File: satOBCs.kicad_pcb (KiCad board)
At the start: 2 copper layers, 55.2 x 94.2 mm, 11 parts, among them J1 Battery power, J2 Conn_01x10_Pin, J3 Conn_01x10_Pin, SW1 SW_Push, U2 mpu-9250, U3 AZ1117-3.3, U6 DHT11

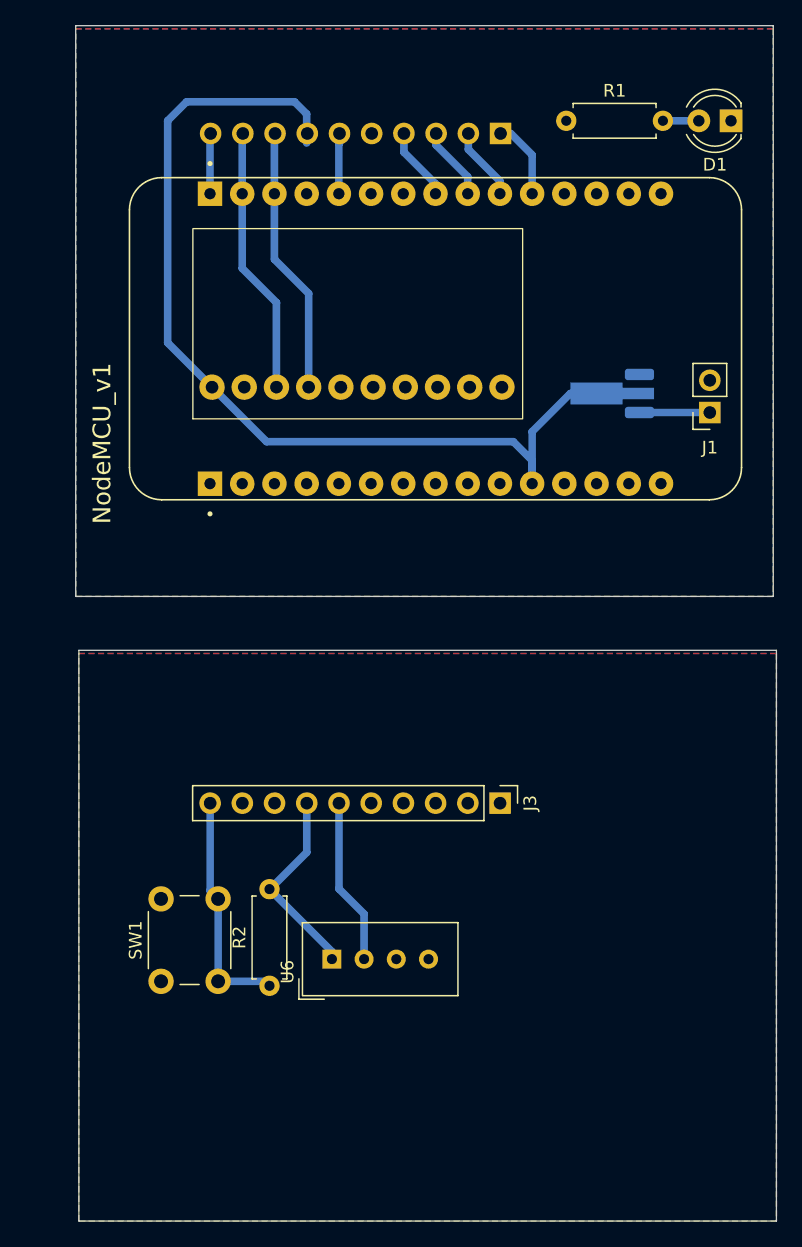
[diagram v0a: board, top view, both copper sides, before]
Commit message: 4th edited
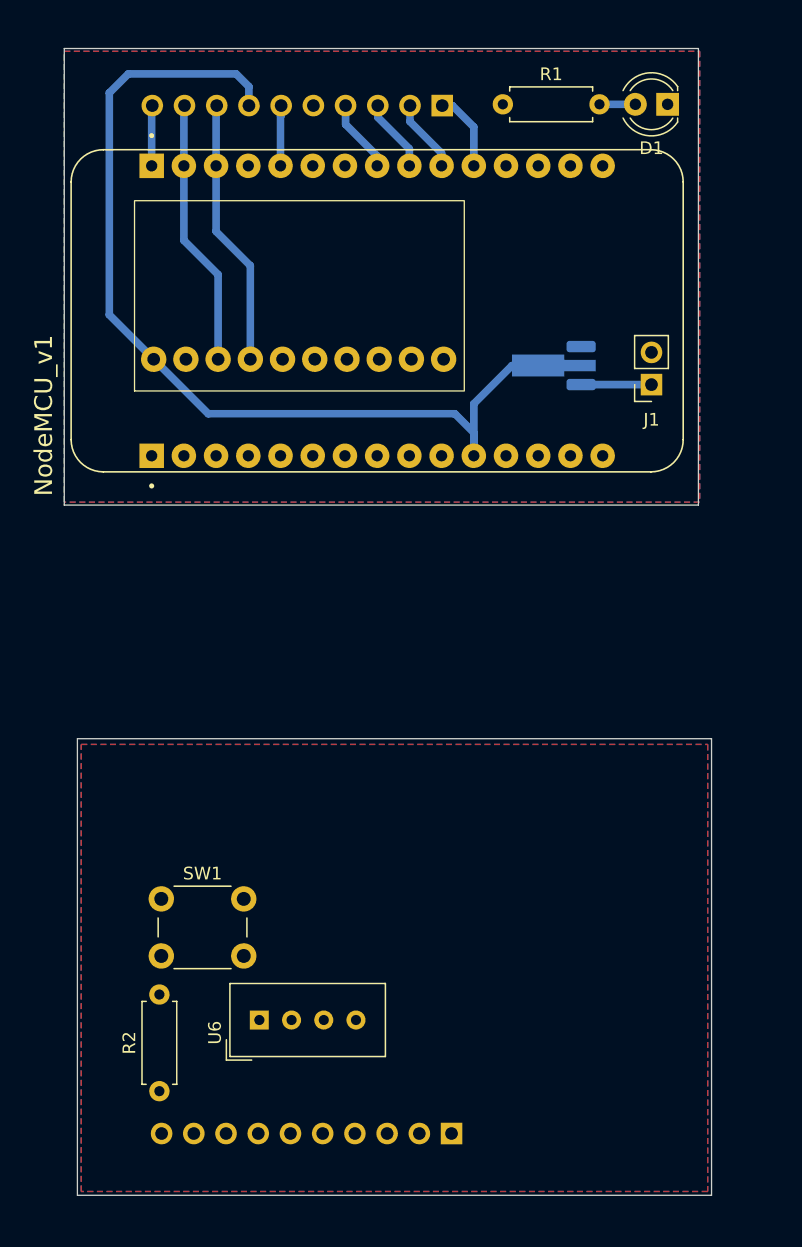
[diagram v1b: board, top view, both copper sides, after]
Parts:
- J3: moved to B.Cu
- moved J3 26.3 mm to (136.6, 133.8), turned to 90 degrees
- moved R2 12.0 mm to (113.6, 130.5)
- moved U6 7.47 mm to (121.5, 124.9)
- moved SW1 6.50 mm to (113.8, 115.3), turned to 0 degrees
- moved D1 5.17 mm to (153.7, 52.7)
- moved R1 5.17 mm to (140.7, 52.7)
- moved U2 5.10 mm to (126.1, 67.8)
- moved J1 5.10 mm to (152.4, 74.8)
- moved J2 5.10 mm to (135.9, 52.8)
- moved NodeMCU_v1 5.10 mm to (130.8, 69.0)
- moved U3 5.10 mm to (144.4, 73.3)
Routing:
- net /RST: track 22.5 -> 4.00 mm
- net +3V3: track 95.5 -> 79.2 mm
- net /DHT_data: track 17.9 -> 4.77 mm
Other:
- board size 55.2 x 94.2 mm -> 51 x 90.4 mm

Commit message: added last
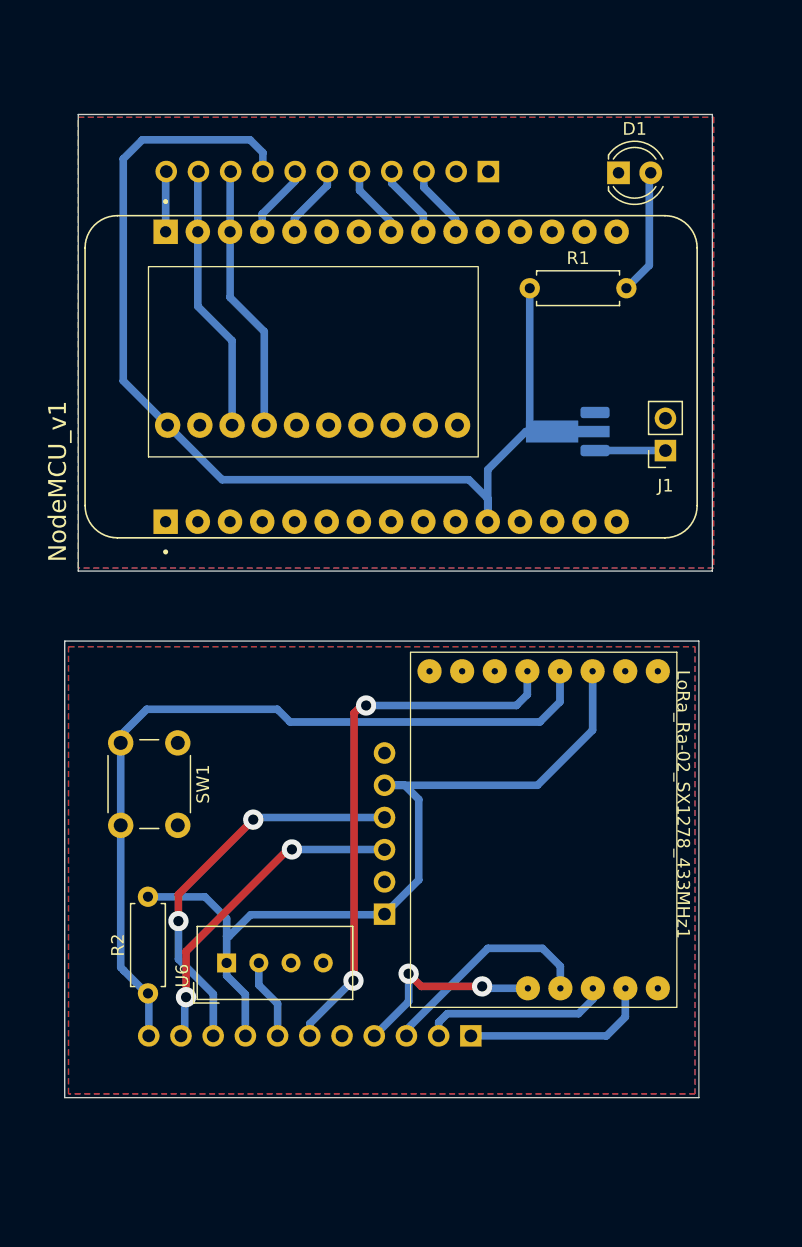
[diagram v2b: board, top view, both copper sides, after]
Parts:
- removed J3: Conn_01x10_Pin, Connector_PinHeader_2.54mm:PinHeader_1x10_P2.54mm_Vertical
- added J4: Conn_01x11_Pin, Connector_PinSocket_2.54mm:PinSocket_1x11_P2.54mm_Vertical, B.Cu at (139.5, 58.0)
- added LoRa_Ra-02_SX1278_433MHz1: ~, prashantkicadlibrary:LORA-02, F.Cu at (154.4, 107.9)
- added U1: BMP280, Connector_PinHeader_2.54mm:PinHeader_1x06_P2.54mm_Vertical, B.Cu at (131.3, 116.5)
- J2: value Conn_01x10_Pin -> Conn_01x11_Pin; footprint Connector_PinHeader_2.54mm:PinHeader_1x10_P2.54mm_Vertical -> Connector_PinSocket_2.54mm:PinSocket_1x11_P2.54mm_Vertical
- moved J2 73.4 mm to (138.2, 126.2)
- moved R1 14.7 mm to (142.8, 67.2)
- moved SW1 12.4 mm to (115.0, 103.0), turned to -90 degrees
- moved R2 7.76 mm to (112.7, 122.8)
- moved D1 6.64 mm to (149.8, 58.1), turned to 0 degrees
- moved J1 5.32 mm to (153.5, 80.0)
- moved NodeMCU_v1 5.32 mm to (131.9, 74.2)
- moved U2 5.32 mm to (127.2, 73.0)
- moved U3 5.32 mm to (145.5, 78.5)
- moved U6 5.19 mm to (118.9, 120.4)
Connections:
- J2 pad 10: /RST -> /SCL
- J2 pad 6: /DHT_data -> /D3
- J2 pad 7: +3V3 -> /DHT_data
- J2 pad 8: /SDA -> +3V3
- J2 pad 9: /SCL -> /SDA
- NodeMCU_v1 pad 26: /DHT_data -> /D3
- NodeMCU_v1 pad 27: /D3 -> /DHT_data
- R1 pad 1: /LED -> +3V3
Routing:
- net +3V3: track 79.2 -> 162.1 mm
- net /RST: track 4.00 -> 67.7 mm
- net /D3: track 0.00 -> 48.9 mm, vias 0 -> 2
- net /SDA: track 20.4 -> 51.4 mm, vias 0 -> 2
- net /SCL: track 20.6 -> 46.4 mm, vias 0 -> 2
- net /MISO: track 5.80 -> 23.4 mm
- net /SCLK: track 5.78 -> 21.7 mm, vias 0 -> 2
- net /MOSI: track 5.78 -> 20.6 mm
- net /CS: track 6.26 -> 15.1 mm
- net /DHT_data: track 4.77 -> 12.2 mm
- net Net-(D1-A): track 2.83 -> 10.0 mm
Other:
- board size 51 x 90.4 mm -> 51.1 x 77.5 mm
